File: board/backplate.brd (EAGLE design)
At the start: 100 x 80 mm, 22 parts, among them IC1 MAX7219CNG, IC2 MAX7219CNG, IC3 MAX7219CNG, IC4 MAX7219CNG

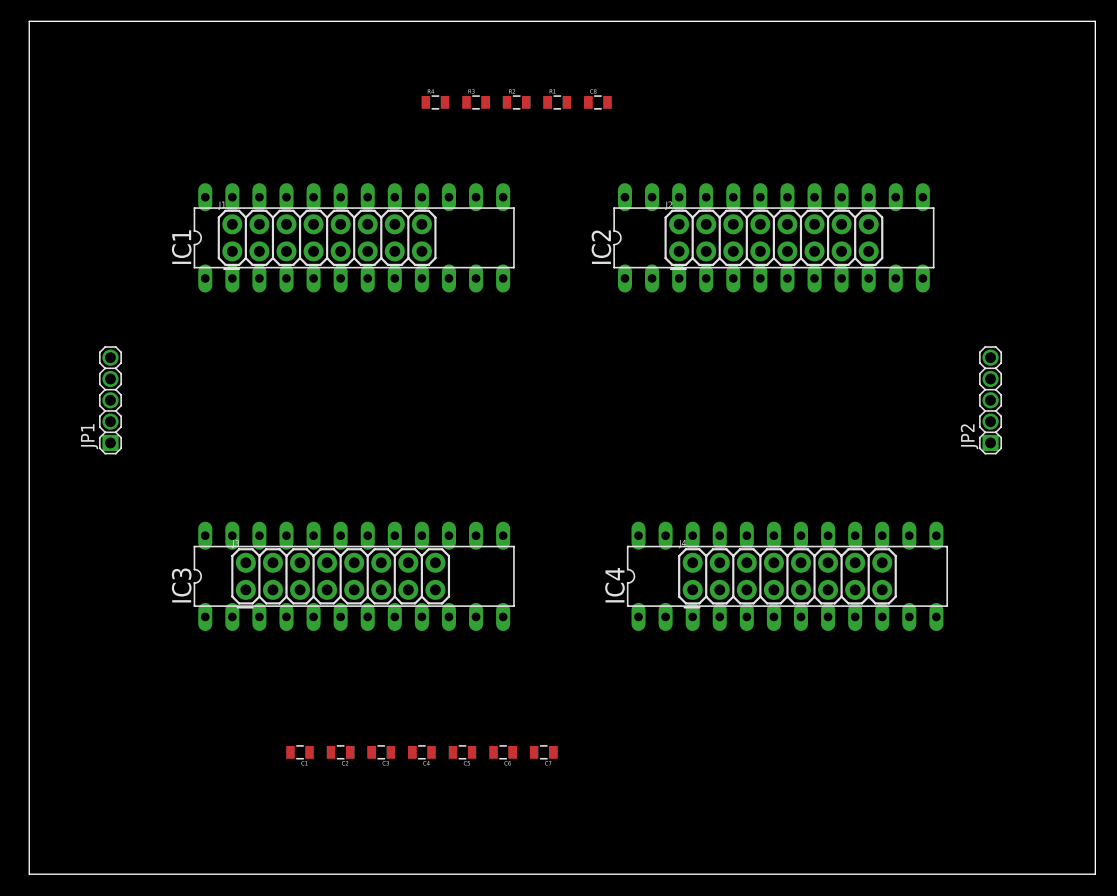
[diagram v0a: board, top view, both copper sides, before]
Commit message: add greber
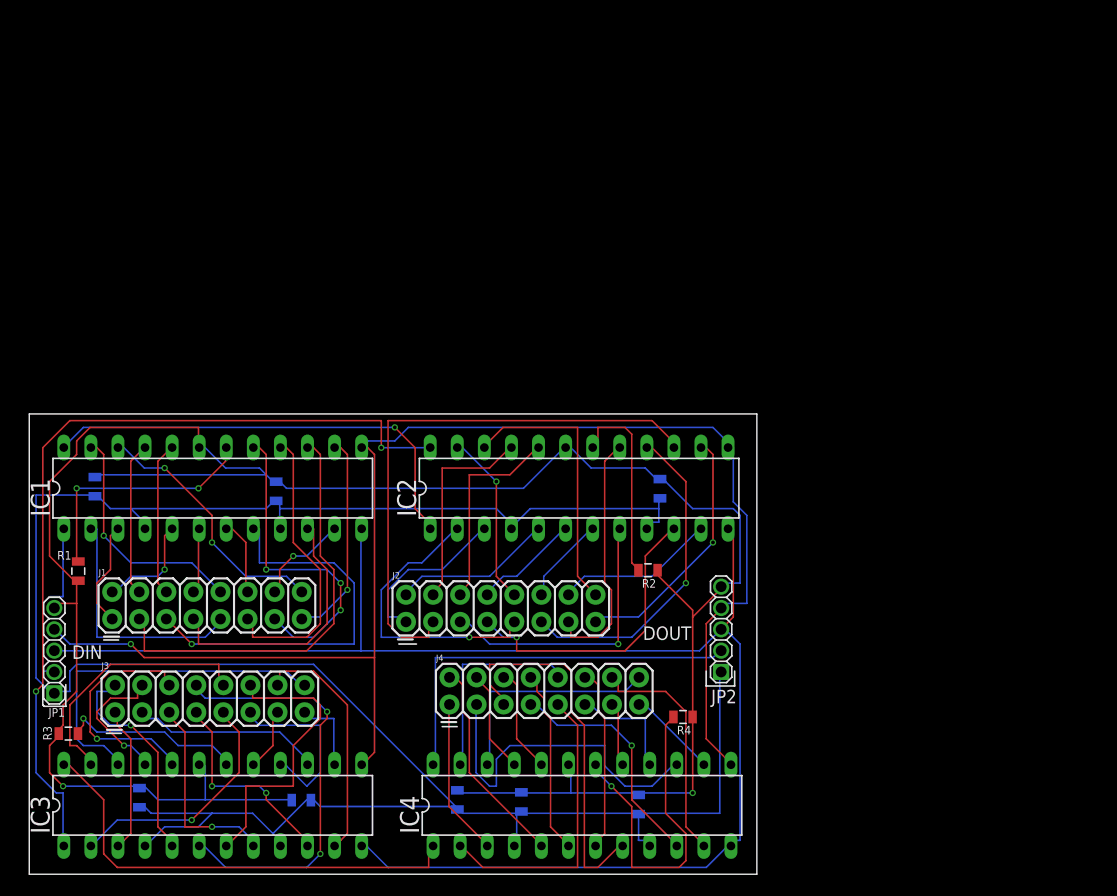
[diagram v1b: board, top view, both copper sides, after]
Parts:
- moved C8 78.1 mm to (10.3, 7.18), flipped to the bottom, turned to 270 degrees
- moved R3 70.5 mm to (3.67, 13.2)
- moved R1 62.9 mm to (4.60, 28.4), turned to 90 degrees
- moved R4 62.1 mm to (61.3, 14.7), turned to 180 degrees
- moved R2 45.6 mm to (58.0, 28.5), turned to 180 degrees
- moved J2 43.2 mm to (35.3, 23.7)
- moved C4 39.5 mm to (6.16, 36.4), flipped to the bottom, turned to 270 degrees
- moved J1 36.3 mm to (7.78, 23.9)
- moved JP2 33.2 mm to (64.9, 23.0)
- moved C5 30.9 mm to (59.2, 36.2), flipped to the bottom, turned to 270 degrees
- moved IC2 29.8 mm to (51.6, 36.2)
- moved IC4 28.9 mm to (51.9, 6.46)
- moved IC1 27.0 mm to (17.2, 36.2)
- moved IC3 25.2 mm to (17.2, 6.46)
- moved J4 25.2 mm to (39.4, 15.9)
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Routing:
- net GND: track 0.00 -> 221.3 mm
- net VCC: track 0.00 -> 211.2 mm, vias 0 -> 2
- net CS: track 0.00 -> 143.4 mm
- net CLK: track 0.00 -> 132.8 mm, vias 0 -> 1
- net N$71: track 0.00 -> 79.0 mm, vias 0 -> 2
- net N$21: track 0.00 -> 53.2 mm
- net N$72: track 0.00 -> 43.5 mm
- net N$70: track 0.00 -> 42.7 mm, vias 0 -> 1
- net N$5: track 0.00 -> 39.9 mm
- net N$51: track 0.00 -> 39.8 mm, vias 0 -> 2
- net N$7: track 0.00 -> 37.7 mm, vias 0 -> 1
- net DOUT: track 0.00 -> 37.2 mm
- net N$57: track 0.00 -> 35.5 mm
- net N$49: track 0.00 -> 33.4 mm
- net N$55: track 0.00 -> 32.3 mm
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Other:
- board size 100 x 80 mm -> 68.2 x 43.2 mm
- board text added: "DIN"
- board text added: "DOUT"
- board text added: "https://github.com/5shekel/monty"
